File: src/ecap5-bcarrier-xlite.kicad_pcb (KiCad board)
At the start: 4 copper layers, 161.3 x 55.2 mm, 55 parts, among them J1 DDR4_SODIMM_Board, J2 DDR4_SODIMM_Board, J3 Conn_01x04, J4 Conn_01x04, J5 USB_C_Receptacle_USB2.0_14P, J6 Conn_Coaxial, J7 Conn_Coaxial, J8 Conn_Coaxial, J9 1935161, Q1 BC846BR13, Q2 BC846BR13, SW1 RESET_SOM1, SW2 RESET_SOM2, SW3 USER1, SW4 USER1, U1 FT232RN, U2 AP7375-33SA-7

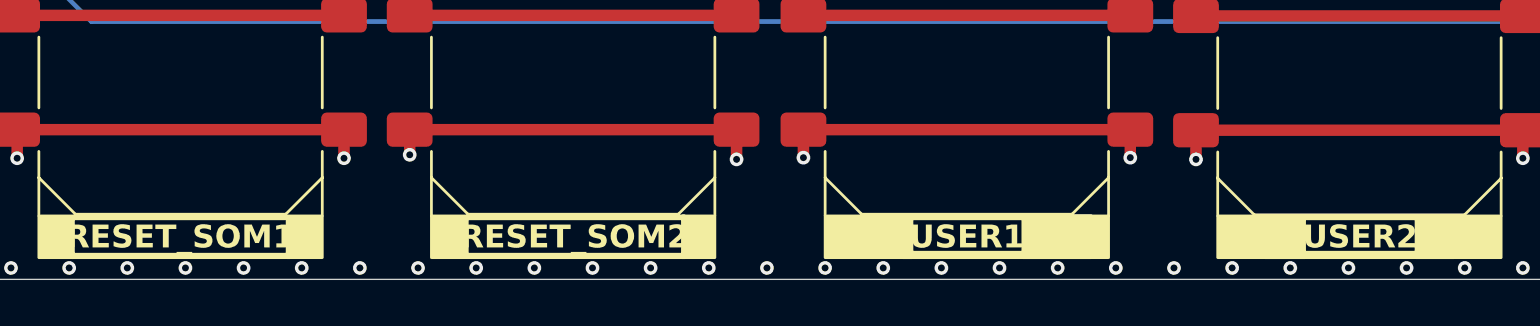
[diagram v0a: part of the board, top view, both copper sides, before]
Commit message: Save button footprint in local library
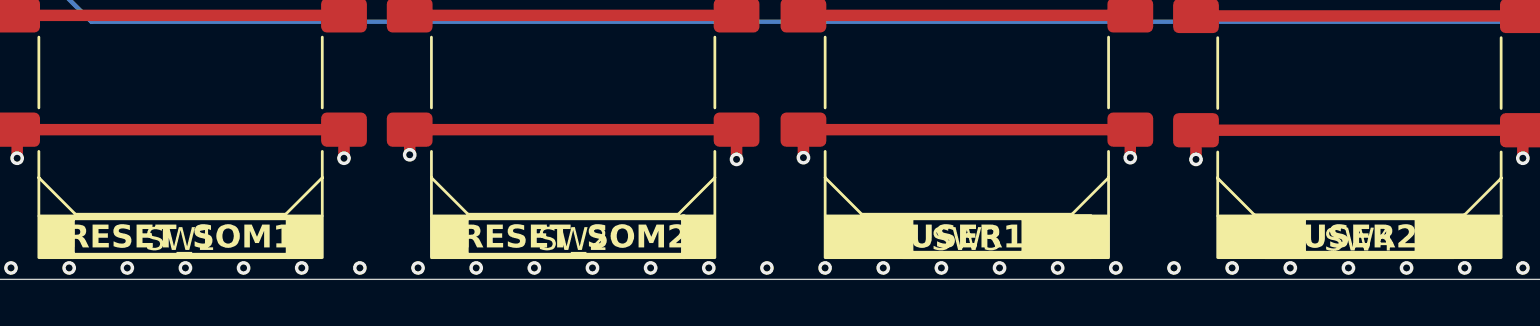
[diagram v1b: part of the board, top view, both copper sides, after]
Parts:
- SW1, SW2, SW3, SW4: footprint Button_Switch_SMD:SW_Push_1P1T_NO_CK_PTS125Sx73SMTR -> ECAP5-BCARRIER-XLITE:SW_Push_1P1T_NO_CK_PTS125Sx73SMTR_1
